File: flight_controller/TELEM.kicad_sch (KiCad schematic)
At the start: 18 parts, among them J11 A1257WV-S-6P-LCP, J12 A1257WV-S-6P-LCP, J13 A1257WV-S-6P-LCP

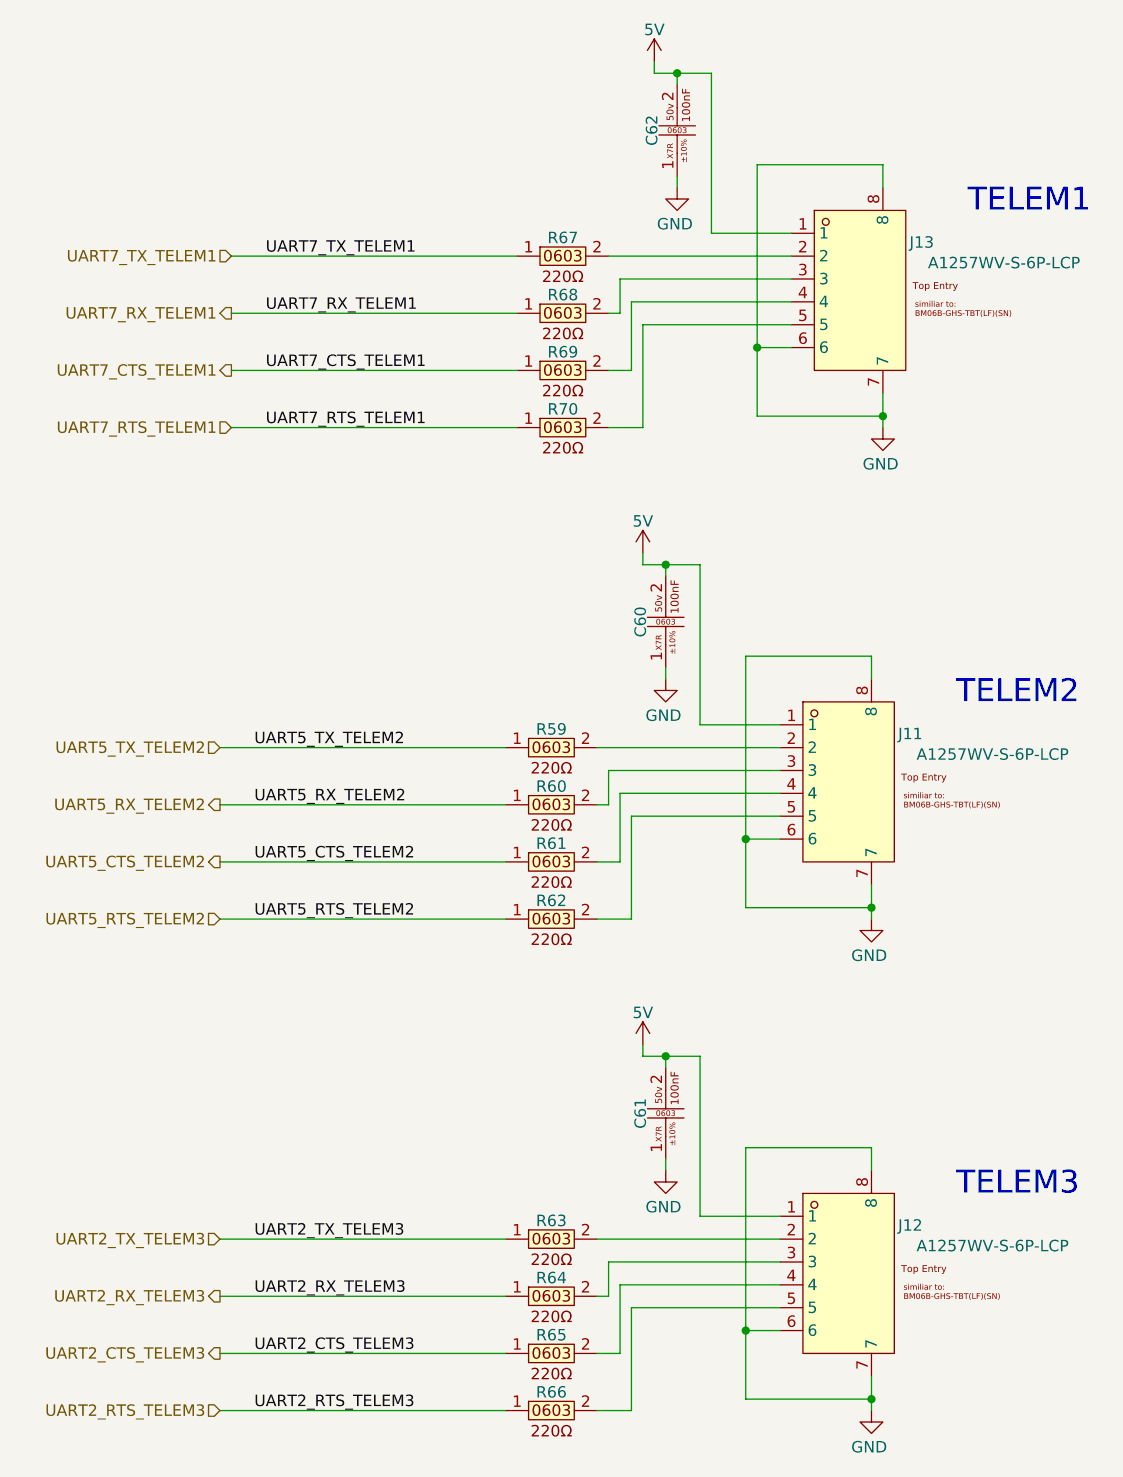
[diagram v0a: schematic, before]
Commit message: Updated power and usb connectors, annotations and netlist check
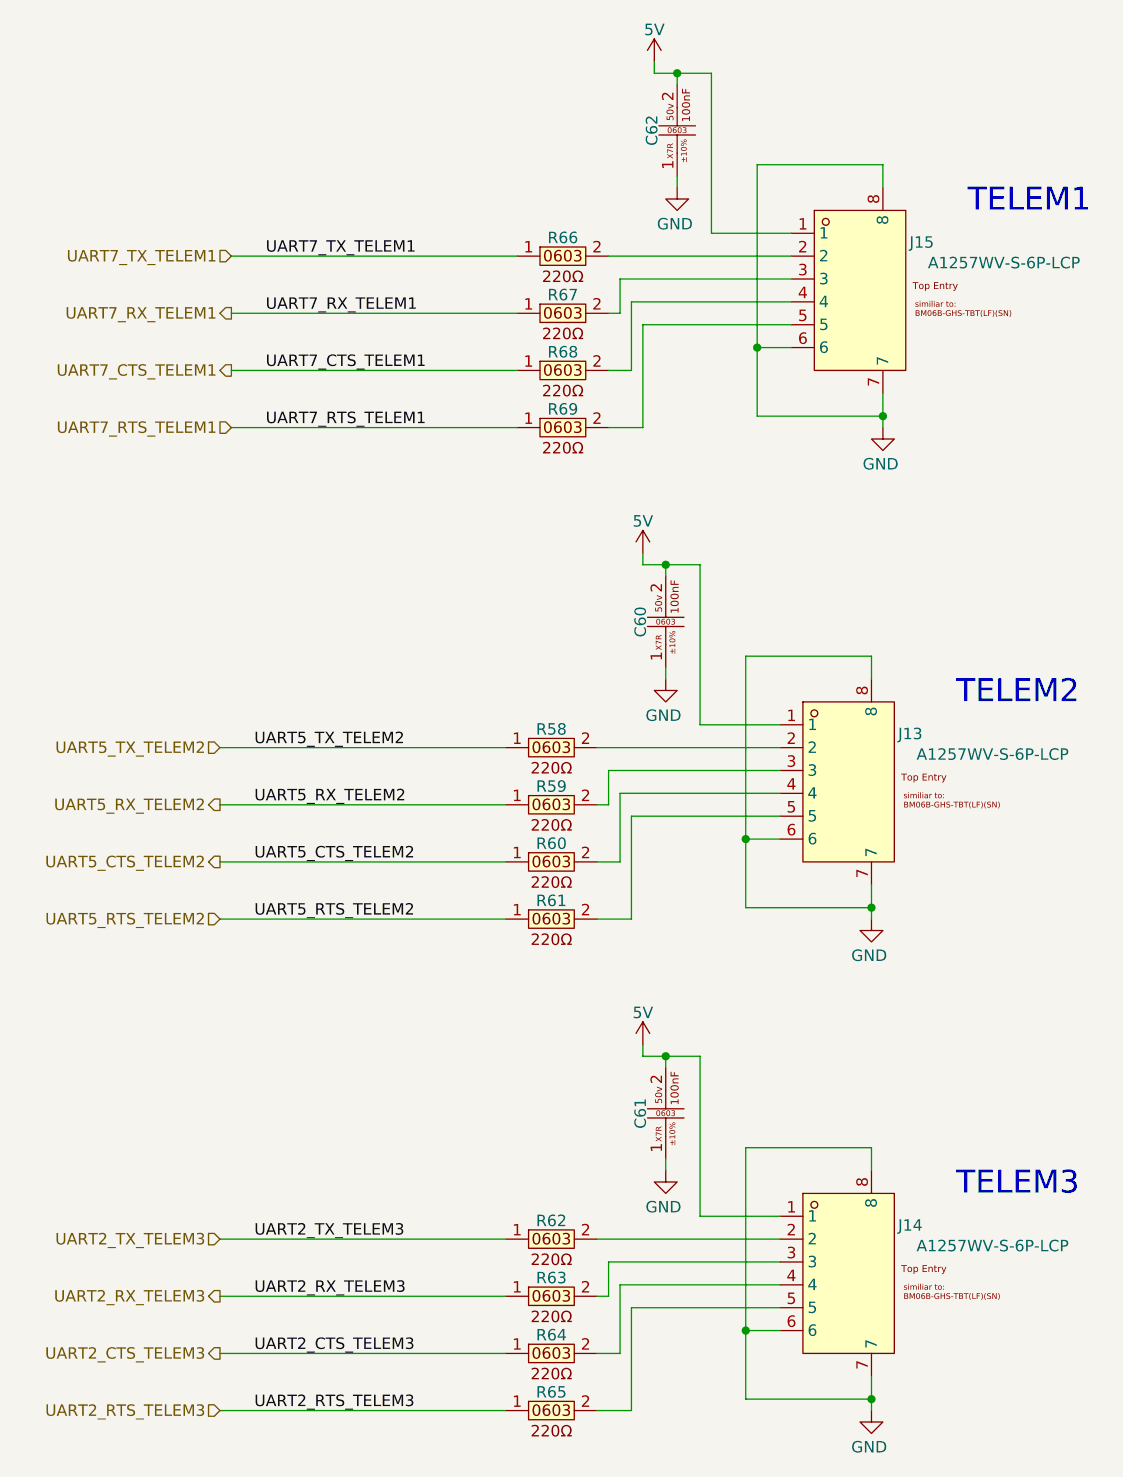
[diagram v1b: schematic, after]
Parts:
- renumbered J11 to J13, J12 to J14, J13 to J15, R59 to R58, R60 to R59, R61 to R60, R62 to R61, R63 to R62, R64 to R63, R65 to R64, R66 to R65, R67 to R66, R68 to R67, R69 to R68, R70 to R69
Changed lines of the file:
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@@
-		(polyline
-			(pts
-				(xy 68.58 129.54) (xy 68.58 181.61) (xy 148.59 181.61) (xy 148.59 129.54)
-			)
-			(stroke
-				(width 0)
-				(type dash)
-			)
-			(fill
-				(type none)
-			)
-		)
-	)
-	(rule_area
 		(polyline
 			(pts
@@
 			(pts
 				(xy 79.375 74.93) (xy 79.375 127) (xy 173.99 127.635) (xy 173.99 74.93)
+			)
+			(stroke
+				(width 0)
+				(type dash)
+			)
+			(fill
+				(type none)
+			)
+		)
+	)
+	(rule_area
+		(polyline
+			(pts
+				(xy 68.58 129.54) (xy 68.58 181.61) (xy 148.59 181.61) (xy 148.59 129.54)
 			)
 			(stroke
@@
 		(dnp no)
 		(fields_autoplaced yes)
-		(property "Reference" "R65"
+		(property "Reference" "R64"
 			(at 85.09 166.878 0)
 			(do_not_autoplace yes)
@@
 			(project "FP_BOARD"
 				(path "/17737359-1a8e-4237-8899-d9604030bc1d/ee742a7d-8184-434b-840f-4020f45cd711"
-					(reference "R65")
+					(reference "R64")
 					(unit 1)
 				)
@@
 		(on_board yes)
 		(dnp no)
-		(property "Reference" "#PWR0160"
+		(property "Reference" "#PWR0158"
 			(at 95.25 138.43 0)
 			(effects
@@
 			(project "FP_BOARD"
 				(path "/17737359-1a8e-4237-8899-d9604030bc1d/ee742a7d-8184-434b-840f-4020f45cd711"
-					(reference "#PWR0160")
+					(reference "#PWR0158")
 					(unit 1)
 				)
@@
 		(dnp no)
 		(fields_autoplaced yes)
-		(property "Reference" "R66"
+		(property "Reference" "R65"
 			(at 85.09 173.228 0)
 			(do_not_autoplace yes)
@@
 			(project "FP_BOARD"
 				(path "/17737359-1a8e-4237-8899-d9604030bc1d/ee742a7d-8184-434b-840f-4020f45cd711"
-					(reference "R66")
+					(reference "R65")
 					(unit 1)
 				)
@@
 		(dnp no)
 		(fields_autoplaced yes)
-		(property "Reference" "R61"
+		(property "Reference" "R60"
 			(at 85.09 112.268 0)
 			(do_not_autoplace yes)
@@
 			(project "FP_BOARD"
 				(path "/17737359-1a8e-4237-8899-d9604030bc1d/ee742a7d-8184-434b-840f-4020f45cd711"
-					(reference "R61")
+					(reference "R60")
 					(unit 1)
 				)
@@
 		(dnp no)
 		(fields_autoplaced yes)
-		(property "Reference" "R63"
+		(property "Reference" "R62"
 			(at 85.09 154.178 0)
 			(do_not_autoplace yes)
@@
 			(project "FP_BOARD"
 				(path "/17737359-1a8e-4237-8899-d9604030bc1d/ee742a7d-8184-434b-840f-4020f45cd711"
-					(reference "R63")
+					(reference "R62")
 					(unit 1)
 				)
@@
 		(dnp no)
 		(fields_autoplaced yes)
-		(property "Reference" "J11"
+		(property "Reference" "J13"
 			(at 124.968 100.076 0)
 			(do_not_autoplace yes)
@@
 			(project "FP_BOARD"
 				(path "/17737359-1a8e-4237-8899-d9604030bc1d/ee742a7d-8184-434b-840f-4020f45cd711"
-					(reference "J11")
+					(reference "J13")
 					(unit 1)
 				)
@@
 		(dnp no)
 		(fields_autoplaced yes)
-		(property "Reference" "J13"
+		(property "Reference" "J15"
 			(at 126.238 45.466 0)
 			(do_not_autoplace yes)
@@
 			(project "FP_BOARD"
 				(path "/17737359-1a8e-4237-8899-d9604030bc1d/ee742a7d-8184-434b-840f-4020f45cd711"
-					(reference "J13")
+					(reference "J15")
 					(unit 1)
 				)
@@
 		(on_board yes)
 		(dnp no)
-		(property "Reference" "#PWR0159"
+		(property "Reference" "#PWR0157"
 			(at 95.25 83.82 0)
 			(effects
@@
 			(project "FP_BOARD"
 				(path "/17737359-1a8e-4237-8899-d9604030bc1d/ee742a7d-8184-434b-840f-4020f45cd711"
-					(reference "#PWR0159")
+					(reference "#PWR0157")
 					(unit 1)
 				)
@@
 		(dnp no)
 		(fields_autoplaced yes)
-		(property "Reference" "J12"
+		(property "Reference" "J14"
 			(at 124.968 154.686 0)
 			(do_not_autoplace yes)
@@
 			(project "FP_BOARD"
 				(path "/17737359-1a8e-4237-8899-d9604030bc1d/ee742a7d-8184-434b-840f-4020f45cd711"
-					(reference "J12")
+					(reference "J14")
 					(unit 1)
 				)
@@
 		(dnp no)
 		(fields_autoplaced yes)
-		(property "Reference" "R64"
+		(property "Reference" "R63"
 			(at 85.09 160.528 0)
 			(do_not_autoplace yes)
@@
 			(project "FP_BOARD"
 				(path "/17737359-1a8e-4237-8899-d9604030bc1d/ee742a7d-8184-434b-840f-4020f45cd711"
-					(reference "R64")
+					(reference "R63")
 					(unit 1)
 				)
@@
 		(dnp no)
 		(fields_autoplaced yes)
-		(property "Reference" "R70"
+		(property "Reference" "R69"
 			(at 86.36 64.008 0)
 			(do_not_autoplace yes)
@@
 			(project "FP_BOARD"
 				(path "/17737359-1a8e-4237-8899-d9604030bc1d/ee742a7d-8184-434b-840f-4020f45cd711"
-					(reference "R70")
+					(reference "R69")
 					(unit 1)
 				)
@@
 		(on_board yes)
 		(dnp no)
-		(property "Reference" "#PWR0163"
+		(property "Reference" "#PWR0161"
 			(at 97.79 154.94 0)
 			(effects
@@
 			(project "FP_BOARD"
 				(path "/17737359-1a8e-4237-8899-d9604030bc1d/ee742a7d-8184-434b-840f-4020f45cd711"
-					(reference "#PWR0163")
+					(reference "#PWR0161")
 					(unit 1)
 				)
@@
 		(dnp no)
 		(fields_autoplaced yes)
-		(property "Reference" "R67"
+		(property "Reference" "R66"
 			(at 86.36 44.958 0)
 			(do_not_autoplace yes)
@@
 			(project "FP_BOARD"
 				(path "/17737359-1a8e-4237-8899-d9604030bc1d/ee742a7d-8184-434b-840f-4020f45cd711"
-					(reference "R67")
+					(reference "R66")
 					(unit 1)
 				)
@@
 		(dnp no)
 		(fields_autoplaced yes)
-		(property "Reference" "R62"
+		(property "Reference" "R61"
 			(at 85.09 118.618 0)
 			(do_not_autoplace yes)
@@
 			(project "FP_BOARD"
 				(path "/17737359-1a8e-4237-8899-d9604030bc1d/ee742a7d-8184-434b-840f-4020f45cd711"
-					(reference "R62")
+					(reference "R61")
 					(unit 1)
 				)
@@
 		(dnp no)
 		(fields_autoplaced yes)
-		(property "Reference" "R59"
+		(property "Reference" "R58"
 			(at 85.09 99.568 0)
 			(do_not_autoplace yes)
@@
 			(project "FP_BOARD"
 				(path "/17737359-1a8e-4237-8899-d9604030bc1d/ee742a7d-8184-434b-840f-4020f45cd711"
-					(reference "R59")
+					(reference "R58")
 					(unit 1)
 				)
@@
 		(on_board yes)
 		(dnp no)
-		(property "Reference" "#PWR0166"
+		(property "Reference" "#PWR0164"
 			(at 120.65 181.61 0)
 			(effects
@@
 			(project "FP_BOARD"
 				(path "/17737359-1a8e-4237-8899-d9604030bc1d/ee742a7d-8184-434b-840f-4020f45cd711"
-					(reference "#PWR0166")
+					(reference "#PWR0164")
 					(unit 1)
 				)
@@
 		(on_board yes)
 		(dnp no)
-		(property "Reference" "#PWR0162"
+		(property "Reference" "#PWR0160"
 			(at 97.79 100.33 0)
 			(effects
@@
 			(project "FP_BOARD"
 				(path "/17737359-1a8e-4237-8899-d9604030bc1d/ee742a7d-8184-434b-840f-4020f45cd711"
-					(reference "#PWR0162")
+					(reference "#PWR0160")
 					(unit 1)
 				)
@@
 		(dnp no)
 		(fields_autoplaced yes)
-		(property "Reference" "R68"
+		(property "Reference" "R67"
 			(at 86.36 51.308 0)
 			(do_not_autoplace yes)
@@
 			(project "FP_BOARD"
 				(path "/17737359-1a8e-4237-8899-d9604030bc1d/ee742a7d-8184-434b-840f-4020f45cd711"
-					(reference "R68")
+					(reference "R67")
 					(unit 1)
 				)
@@
 		(dnp no)
 		(fields_autoplaced yes)
-		(property "Reference" "R69"
+		(property "Reference" "R68"
 			(at 86.36 57.658 0)
 			(do_not_autoplace yes)
@@
 			(project "FP_BOARD"
 				(path "/17737359-1a8e-4237-8899-d9604030bc1d/ee742a7d-8184-434b-840f-4020f45cd711"
-					(reference "R69")
+					(reference "R68")
 					(unit 1)
 				)
@@
 		(on_board yes)
 		(dnp no)
-		(property "Reference" "#PWR0165"
+		(property "Reference" "#PWR0163"
 			(at 120.65 127 0)
 			(effects
@@
 			(project "FP_BOARD"
 				(path "/17737359-1a8e-4237-8899-d9604030bc1d/ee742a7d-8184-434b-840f-4020f45cd711"
-					(reference "#PWR0165")
+					(reference "#PWR0163")
 					(unit 1)
 				)
@@
 		(dnp no)
 		(fields_autoplaced yes)
-		(property "Reference" "R60"
+		(property "Reference" "R59"
 			(at 85.09 105.918 0)
 			(do_not_autoplace yes)
@@
 			(project "FP_BOARD"
 				(path "/17737359-1a8e-4237-8899-d9604030bc1d/ee742a7d-8184-434b-840f-4020f45cd711"
-					(reference "R60")
+					(reference "R59")
 					(unit 1)
 				)
@@
 		(on_board yes)
 		(dnp no)
-		(property "Reference" "#PWR0164"
+		(property "Reference" "#PWR0162"
 			(at 99.06 45.72 0)
 			(effects
@@
 			(project "FP_BOARD"
 				(path "/17737359-1a8e-4237-8899-d9604030bc1d/ee742a7d-8184-434b-840f-4020f45cd711"
-					(reference "#PWR0164")
+					(reference "#PWR0162")
 					(unit 1)
 				)
@@
 		(on_board yes)
 		(dnp no)
-		(property "Reference" "#PWR0161"
+		(property "Reference" "#PWR0159"
 			(at 96.52 29.21 0)
 			(effects
@@
 			(project "FP_BOARD"
 				(path "/17737359-1a8e-4237-8899-d9604030bc1d/ee742a7d-8184-434b-840f-4020f45cd711"
-					(reference "#PWR0161")
+					(reference "#PWR0159")
 					(unit 1)
 				)
@@
 		(on_board yes)
 		(dnp no)
-		(property "Reference" "#PWR0167"
+		(property "Reference" "#PWR0165"
 			(at 121.92 72.39 0)
 			(effects
@@
 			(project "FP_BOARD"
 				(path "/17737359-1a8e-4237-8899-d9604030bc1d/ee742a7d-8184-434b-840f-4020f45cd711"
-					(reference "#PWR0167")
-					(unit 1)
-				)
+					(reference "#PWR0165")
+					(unit 1)
+				)
